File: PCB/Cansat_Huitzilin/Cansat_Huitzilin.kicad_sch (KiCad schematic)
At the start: 0 parts

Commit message: Actualización de la PCB
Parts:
- added C1: 10uf, Capacitor_SMD:C_0603_1608Metric, symbol Device:C
- added C10, C11, C12, C9: 22uF, Capacitor_SMD:C_0603_1608Metric, symbol Device:C
- added C13, C14, C2: 10uF, Capacitor_SMD:C_0603_1608Metric, symbol Device:C
- added C15, C17, C18, C19, C20, C22, C23, C3, C5, C8: 100nF, Capacitor_SMD:C_0603_1608Metric, symbol Device:C
- added C16: 1uF, Capacitor_SMD:C_0603_1608Metric, symbol Device:C
- added C21: 2.2uF, Capacitor_SMD:C_0603_1608Metric, symbol Device:C
- added C25, C26: C_Polarized, Capacitor_SMD:CP_Elec_6.3x5.8, symbol Device:C_Polarized
- added C4, C7: 10nF, Capacitor_SMD:C_0603_1608Metric, symbol Device:C
- added C6: 2.7nF, Capacitor_SMD:C_0603_1608Metric, symbol Device:C
- added D1: D_Schottky, Diode_SMD:D_SOD-123F, symbol Device:D_Schottky
- added H1, H2, H3, H4: MountingHole_Pad, MountingHole:MountingHole_3.2mm_M3, symbol Mechanical:MountingHole_Pad
- added IC1: AP64501SP-13, Package_SO:SOIC-8-1EP_3.9x4.9mm_P1.27mm_EP2.29x3mm, symbol AP64501SP-13:AP64501SP-13
- added IC2: 114993390, 114993390, symbol SamacSys_Parts:114993390
- added IC3: BMM350, BGA9C40P3X3_128X128X54, symbol SamacSys_Parts:BMM350
- added IC4: BMI323, BMI323, symbol SamacSys_Parts:BMI323
- added IC5: STCC4-D-R3, STCC4DR3, symbol SamacSys_Parts:STCC4-D-R3
- added IC6: SHT40-AD1B-R2, SHT40AD1BR2, symbol SamacSys_Parts:SHT40-AD1B-R2
- added J1: Screw_Terminal_01x02, TerminalBlock:TerminalBlock_MaiXu_MX126-5.0-02P_1x02_P5.00mm, symbol Connector:Screw_Terminal_01x02
- added J2: Conn_01x04, Connector_PinHeader_2.54mm:PinHeader_1x04_P2.54mm_Vertical, symbol Connector_Generic:Conn_01x04
- added J3, J5: Conn_01x03, Connector_PinHeader_2.54mm:PinHeader_1x03_P2.54mm_Vertical, symbol Connector_Generic:Conn_01x03
- added J4: Conn_01x06, SM06BPASSTBTLFSN, symbol Connector_Generic:Conn_01x06
- added J6: 503398-1892, 5033981892, symbol SamacSys_Parts:503398-1892
- added L1: 3.3uH, Inductor_SMD:L_Wuerth_WE-PD-Typ-LS, symbol Device:L_Ferrite
- added L2: 10uH, Inductor_SMD:L_1210_3225Metric_Pad1.42x2.65mm_HandSolder, symbol Device:L_Ferrite
- added LS1: MLT-8530, MLT8530, symbol SamacSys_Parts:MLT-8530
- added PS1: LD39200DPUR, SON80P400X400X100-9N-D, symbol SamacSys_Parts:LD39200DPUR
- added Q1: NPN, Package_TO_SOT_SMD:SOT-23, symbol Simulation_SPICE:NPN
- added R1: 100k, Resistor_SMD:R_0603_1608Metric, symbol Device:R_US
- added R10, R12, R13, R14, R15, R16, R17, R5, R9: 10k, Resistor_SMD:R_0603_1608Metric, symbol Device:R_US
- added R11: 1k, Resistor_SMD:R_0603_1608Metric, symbol Device:R_US
- added R2: 15.8k, Resistor_SMD:R_0603_1608Metric, symbol Device:R_US
- added R3: 2.2k, Resistor_SMD:R_0603_1608Metric, symbol Device:R_US
- added R4: 8.87k, Resistor_SMD:R_0603_1608Metric, symbol Device:R_US
- added R6, R7: 4.7k, Resistor_SMD:R_0603_1608Metric, symbol Device:R_US
- added R8: 56k, Resistor_SMD:R_0603_1608Metric, symbol Device:R_US
- added S1, S2: PTS526SM15SMTR2_LFS, PTS526SM15SMTR2LFS, symbol SamacSys_Parts:PTS526SM15SMTR2_LFS
- added SW1: SW_Wuerth_450301014042, Button_Switch_THT:SW_Slide-03_Wuerth-WS-SLTV_10x2.5x6.4_P2.54mm, symbol Switch:SW_Wuerth_450301014042
- added TP1, TP2: TestPoint, TestPoint:TestPoint_Pad_D1.0mm, symbol Connector:TestPoint
- added U1: ESP32-S3-MINI-1U, RF_Module:ESP32-S2-MINI-1U, symbol RF_Module:ESP32-S3-MINI-1U
- added U3: BMP581, BMP581, symbol SamacSys_Parts:BMP581
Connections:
- new net: J6.8 (DAT1), R16.1
- new net: IC1.3 (EN), R1.2, TP1.1
- new net: C10.1, C11.1, C7.2, C8.1, C9.1, L1.2, L2.1, R4.1
- new net: PS1.3 (ADJ/SENSE), R8.1, R9.2
- new net: PS1.5 (PG), TP2.1
- new net: C4.1, IC1.4 (SS)
- new net: D1.2 (A), LS1.3 (-LEAD), Q1.1 (C)
- new net: C5.1, IC1.1 (BST)
- new net: C7.1, IC1.5 (FB), R3.2, R4.2
- new net: IC1.6 (COMP), R2.2
- new net: C5.2, IC1.8 (SW), L1.1
- new net: C6.1, R2.1
- new net: J6.1 (DAT2), R17.1
- new net: Q1.2 (B), R11.2
- new net: C21.1, IC3.C2 (CRST)
- new net: IC5.2 (SDA_C), IC6.1 (SDA)
- new net +3.3V: C14.1, C15.1, C17.1, C18.1, C19.1, C20.1, C22.2, C23.1, IC2.8 (VCC), IC3.B3 (VDDIO), IC3.C1 (VDD), IC4.12 (CSB), IC4.5 (VDDIO), IC4.8 (VDD), IC5.6 (VDDIO), IC5.7 (VDD), IC6.3 (VDD), J2.4 (Pin_4), J6.4 (VDD), PS1.1 (OUT_1), PS1.2 (OUT_2), R10.2, R12.1, R13.2, R14.2, R15.2, R16.2, R17.2, R5.2, R6.1, R7.1, R8.2, U1.3 (3V3), U3.1 (VDDIO), U3.10 (VDD), U3.6 (CSB)
- new net +4V: C12.1, C13.1, C25.1, C26.1, D1.1 (K), J3.2 (Pin_2), J4.3 (Pin_3), J5.2 (Pin_2), L2.2, LS1.2 (+LEAD), PS1.6 (EN), PS1.7 (IN_1), PS1.8 (IN_2)
- new net +9V: J1.1 (Pin_1), SW1.1 (B)
- new net BOOT: R12.2, S2.1 (COM_1), U1.4 (IO0)
- new net BUSY: IC2.11 (BUSY), U1.13 (IO9)
- new net BUZZER: R11.1, U1.38 (IO42)
- new net CS_SD: J6.2 (CD/DAT3), R10.1, U1.37 (IO41)
- new net DIO1: IC2.12 (DIO1), U1.18 (IO14)
- new net Enable ESP: C16.1, R5.1, S1.1 (COM_1), U1.45 (EN)
- new net GND: C1.2, C10.2, C11.2, C12.2, C13.2, C14.2, C15.2, C16.2, C17.2, C18.2, C19.2, C2.2, C20.2, C21.2, C22.1, C23.2, C25.2, C26.2, C3.2, C4.2, C6.2, C8.2, C9.2, H1.1, H2.1, H3.1, H4.1, IC1.7 (GND), IC1.9 (EP), IC2.10 (GND_2), IC2.7 (GND_1), IC3.B1 (GND), IC3.B2 (ADSEL), IC3.C3 (BYPASS), IC4.1 (SDO), IC4.6 (GNDIO), IC4.7 (GND), IC5.3 (ADDR), IC5.4 (VSS), IC6.4 (VSS), J1.2 (Pin_2), J2.1 (Pin_1), J3.1 (Pin_1), J4.4 (Pin_4), J5.1 (Pin_1), J6.11, J6.12, J6.13, J6.14, J6.6 (VSS), PS1.4 (GND_1), PS1.9 (GND_2), Q1.3 (E), R3.1, R9.1, S1.3 (NO_1), S2.3 (NO_1), U1.1 (GND), U1.2 (GND), U1.42 (GND), U1.43 (GND), U1.46 (GND), U1.47 (GND), U1.48 (GND), U1.49 (GND), U1.50 (GND), U1.51 (GND), U1.52 (GND), U1.53 (GND), U1.54 (GND), U1.55 (GND), U1.56 (GND), U1.57 (GND), U1.58 (GND), U1.59 (GND), U1.60 (GND), U1.61 (GND), U1.62 (GND), U1.63 (GND), U1.64 (GND), U1.65 (GND), U3.3 (VSS_1), U3.5 (SDO), U3.8 (VSS_2), U3.9 (VSS_3)
- new net MISO: IC2.2 (MISO), J6.7 (DAT0), R15.1, U1.17 (IO13)
- new net MOSI: IC2.3 (MOSI), J6.3 (CMD), R13.1, U1.15 (IO11)
- new net NRST: IC2.5 (NRST), U1.25 (IO21)
- new net NSS: IC2.6 (NSS), U1.14 (IO10)
- new net RF_SW: IC2.1 (RF_SW_), U1.36 (IO40)
- new net RX: J2.2 (Pin_2), U1.40 (RXD0)
- new net RX_GPS: J4.5 (Pin_5), U1.21 (IO17)
- new net SCK: IC2.4 (SCK), J6.5 (CLK), R14.1, U1.16 (IO12)
- new net SCL: IC3.A3 (SCK), IC4.13 (SCX), IC5.1 (SCL), R7.2, U1.6 (IO2), U3.2 (SCK)
- new net SCL_SHT4: IC5.8 (SCL_C), IC6.2 (SCL)
- new net SDA: IC3.A2 (SDA), IC4.14 (SDX), IC5.5 (SDA), R6.2, U1.5 (IO1), U3.4 (SDI)
- new net SERVO 1: J3.3 (Pin_3), U1.8 (IO4)
- new net SERVO 2: J5.3 (Pin_3), U1.9 (IO5)
- new net Sw_9v: C1.1, C2.1, C3.1, IC1.2 (VIN), R1.1, SW1.3 (A)
- new net TX: J2.3 (Pin_3), U1.39 (TXD0)
- new net TX_GPS: J4.6 (Pin_6), U1.22 (IO18)
- no-connect marks 0 -> 20
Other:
- note added: "BMI-323"
- note added: "BMP-581"
- note added: "Buzzer"
- note added: "COMUNICACION"
- note added: "Conector"
- note added: "DC-DC BUCK 4V OUT"
- note added: "Enable ESP32"
- note added: "GPS UART"
- note added: "I2C BUS"
- note added: "LECTOR SD"
- note added: "LIS2MDL"
- note added: "PROGRAMACION POR UART"
- note added: "Regulador Lineal 4v a 3.3v"
- note added: "SERVOS"
- note added: "STCC4"
- note added: "SWITCH 9V"
- company: (none) -> S.T.R.I.K.E.
- title: (none) -> Cansat

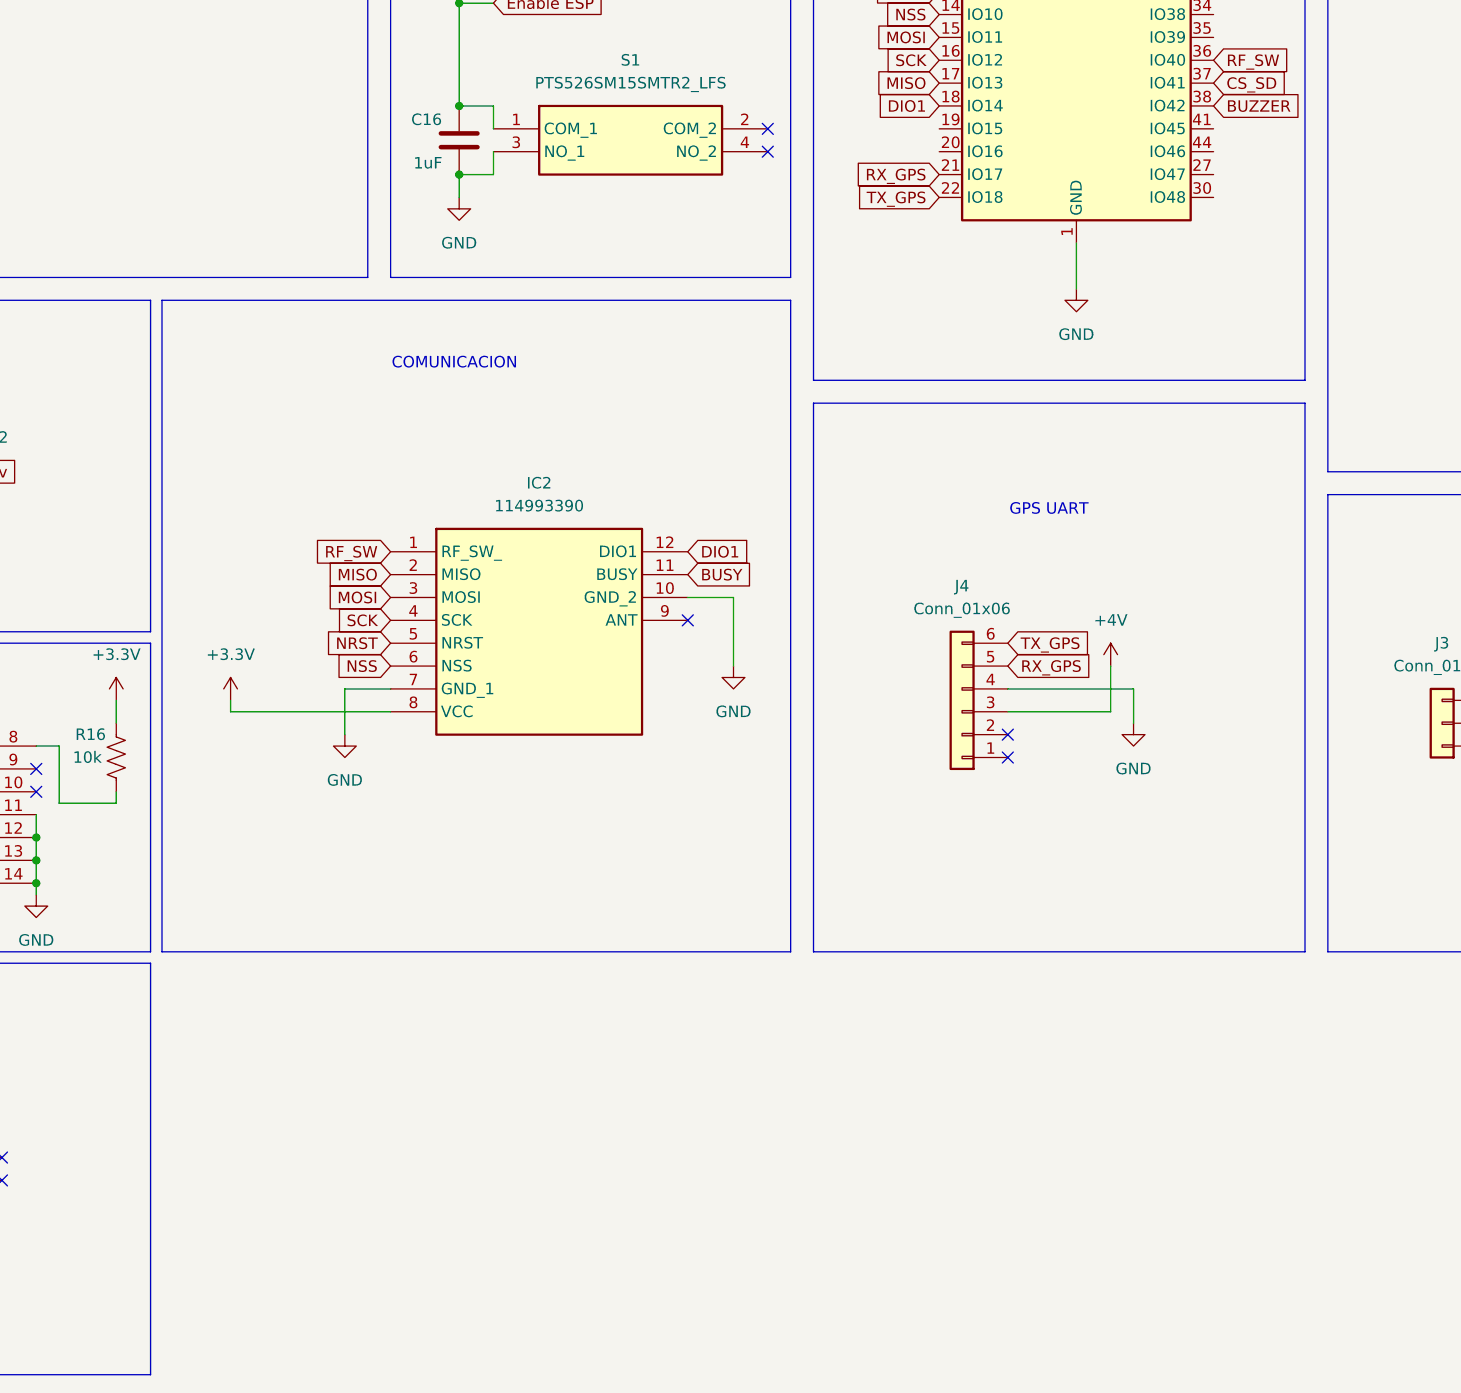
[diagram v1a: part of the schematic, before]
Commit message: Actualización del diseño PCB
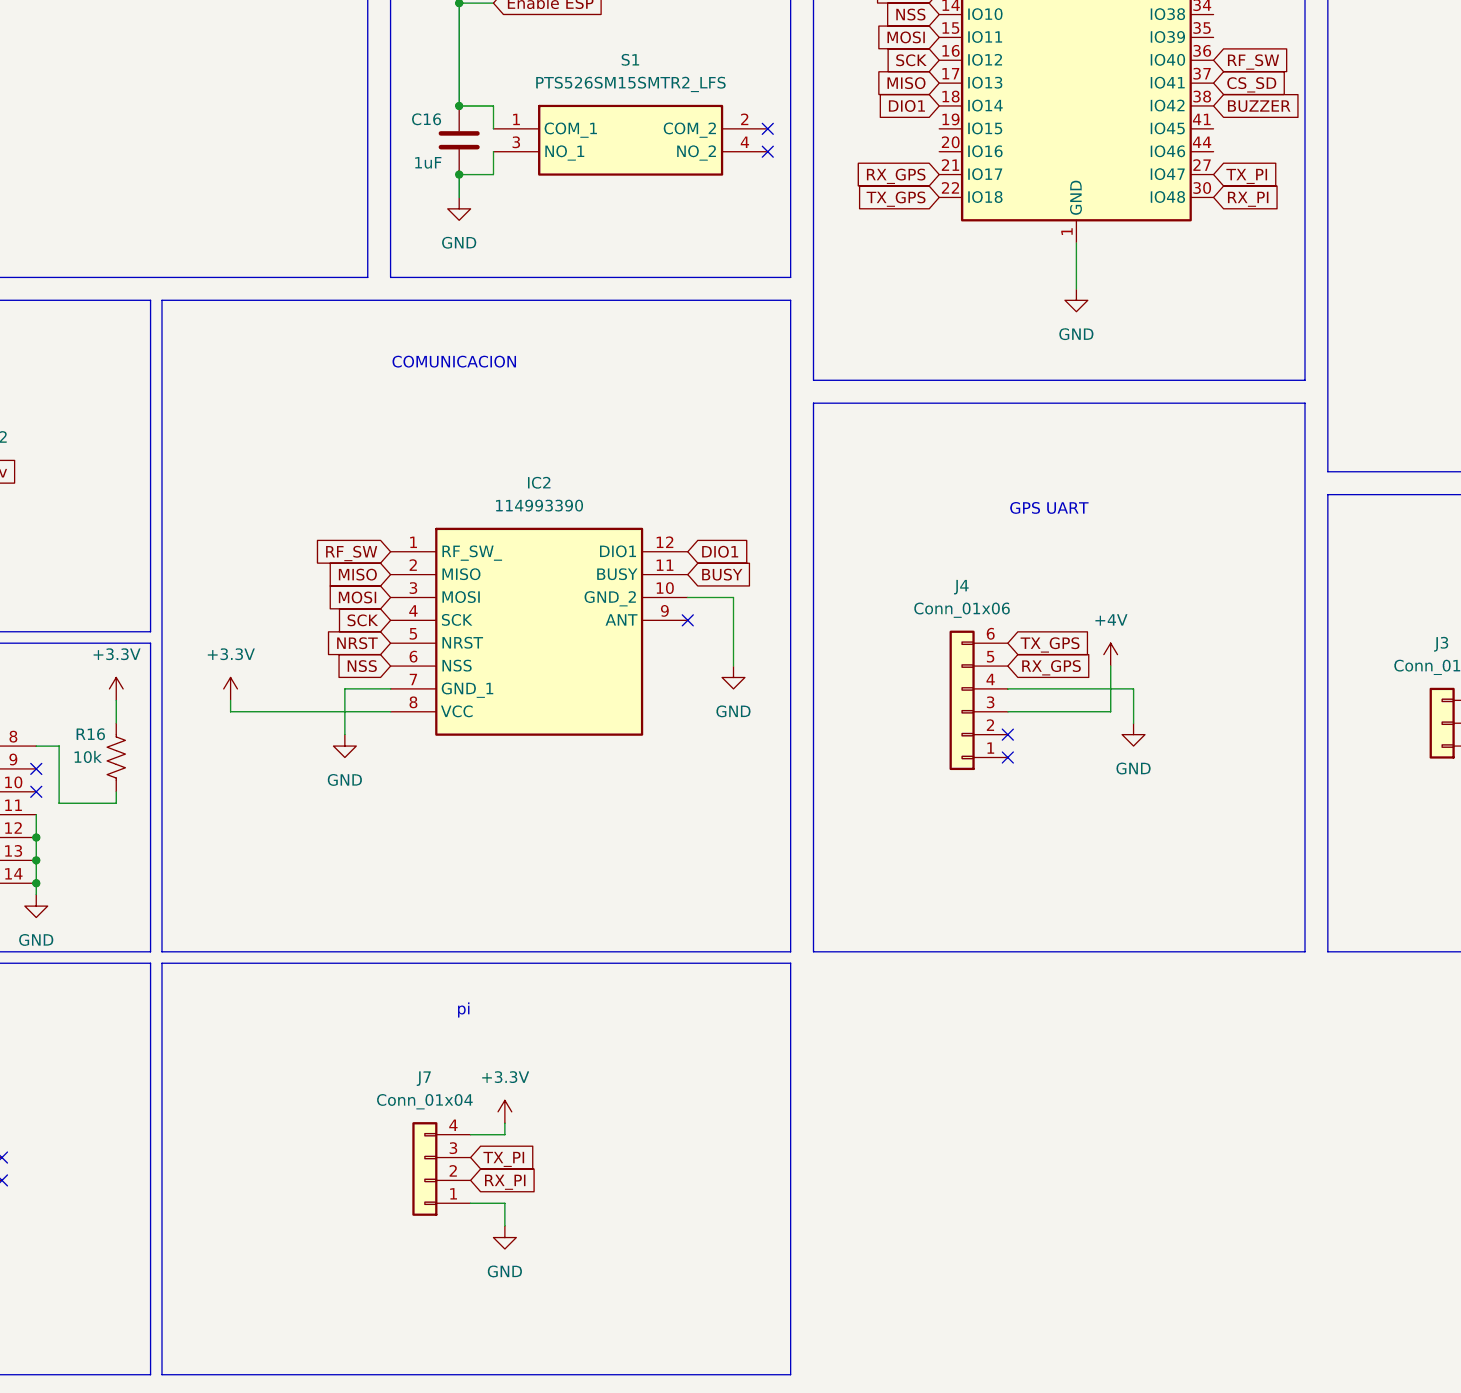
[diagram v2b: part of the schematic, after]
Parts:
- added J7: Conn_01x04, Connector_PinHeader_2.54mm:PinHeader_1x04_P2.54mm_Vertical, symbol Connector_Generic:Conn_01x04
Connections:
- net +3.3V: now also J7.4 (Pin_4)
- net GND: now also J7.1 (Pin_1)
- net TX_PI: now reaches U1.27 (IO47)
- net TX_PI: now also J7.3 (Pin_3)
- net RX_PI: now reaches U1.30 (IO48)
- net RX_PI: now also J7.2 (Pin_2)
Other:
- note added: "pi"
